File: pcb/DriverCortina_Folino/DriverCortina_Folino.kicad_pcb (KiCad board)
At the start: 2 copper layers, 90 x 50 mm, 35 parts, among them J1 AC 220v, J2 Llave Inversora, J3 Motor 1, J4 Motor 2, K1 G3MB-202PL-DC5, K2 G3MB-202PL-DC5, Q1 BC558, Q2 BC558

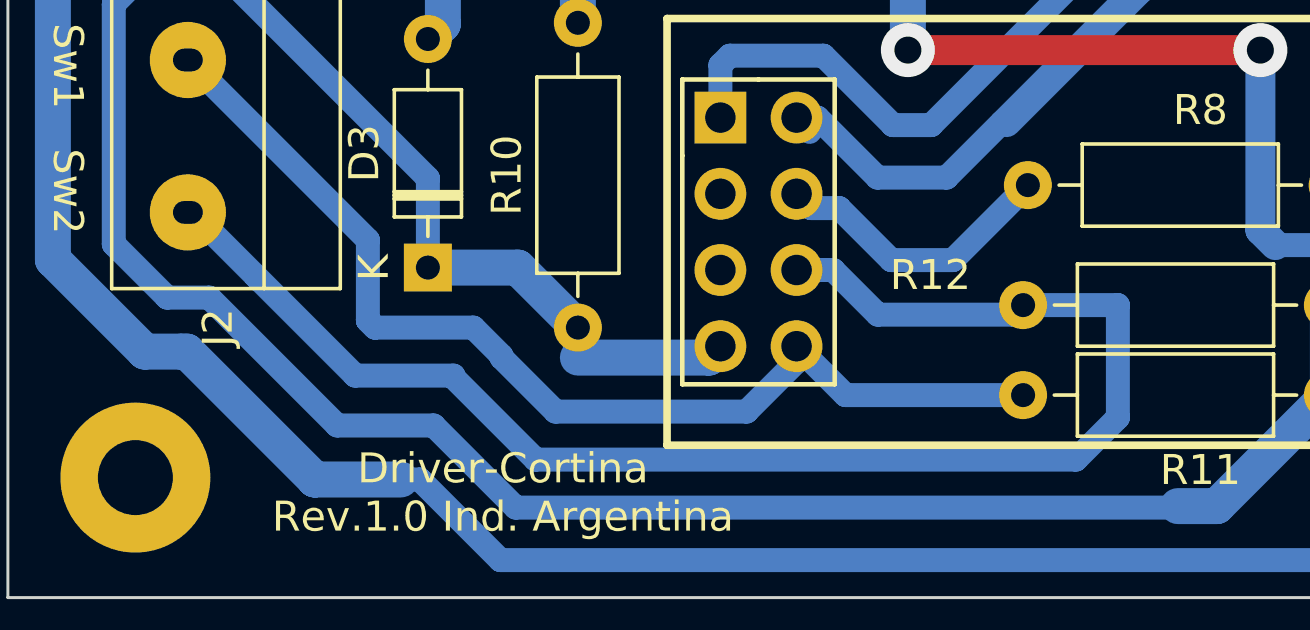
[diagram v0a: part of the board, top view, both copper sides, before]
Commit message: Mejoras de PCB
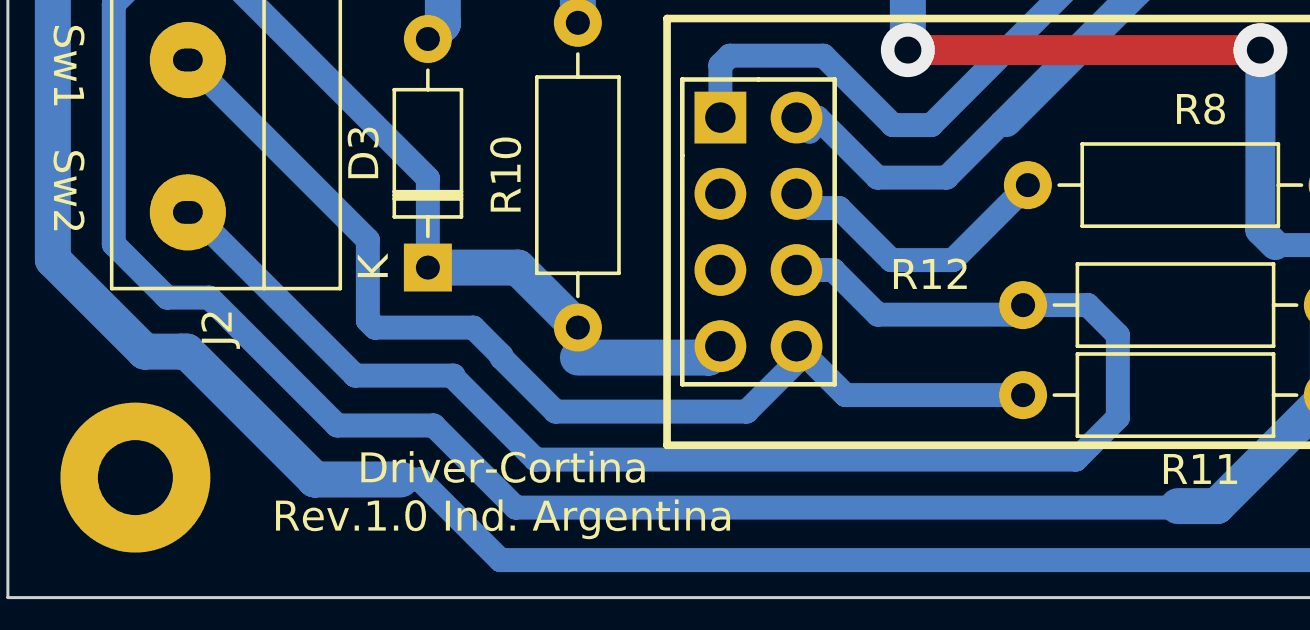
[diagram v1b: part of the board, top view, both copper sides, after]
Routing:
- net /Llave1: track 50.2 -> 49.7 mm
